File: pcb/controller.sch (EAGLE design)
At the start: 20 parts, among them J2 AVR_SPI_PROG_3X22X3_LOCK, Q1 ECS-160-20-3X-TR, U2 32U4

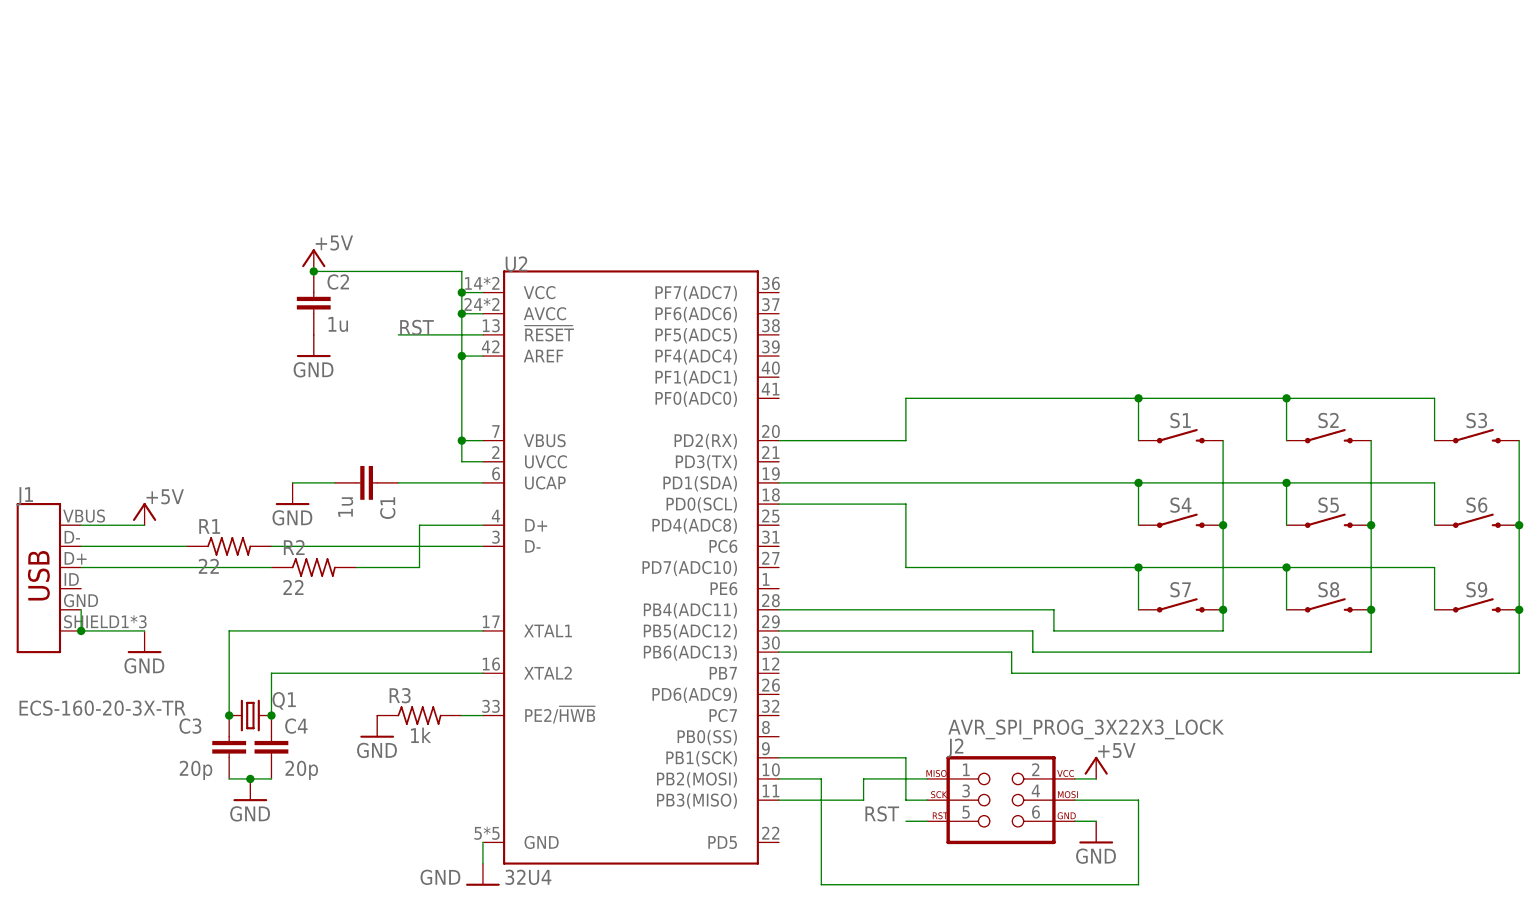
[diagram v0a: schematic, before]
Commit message: finish controller
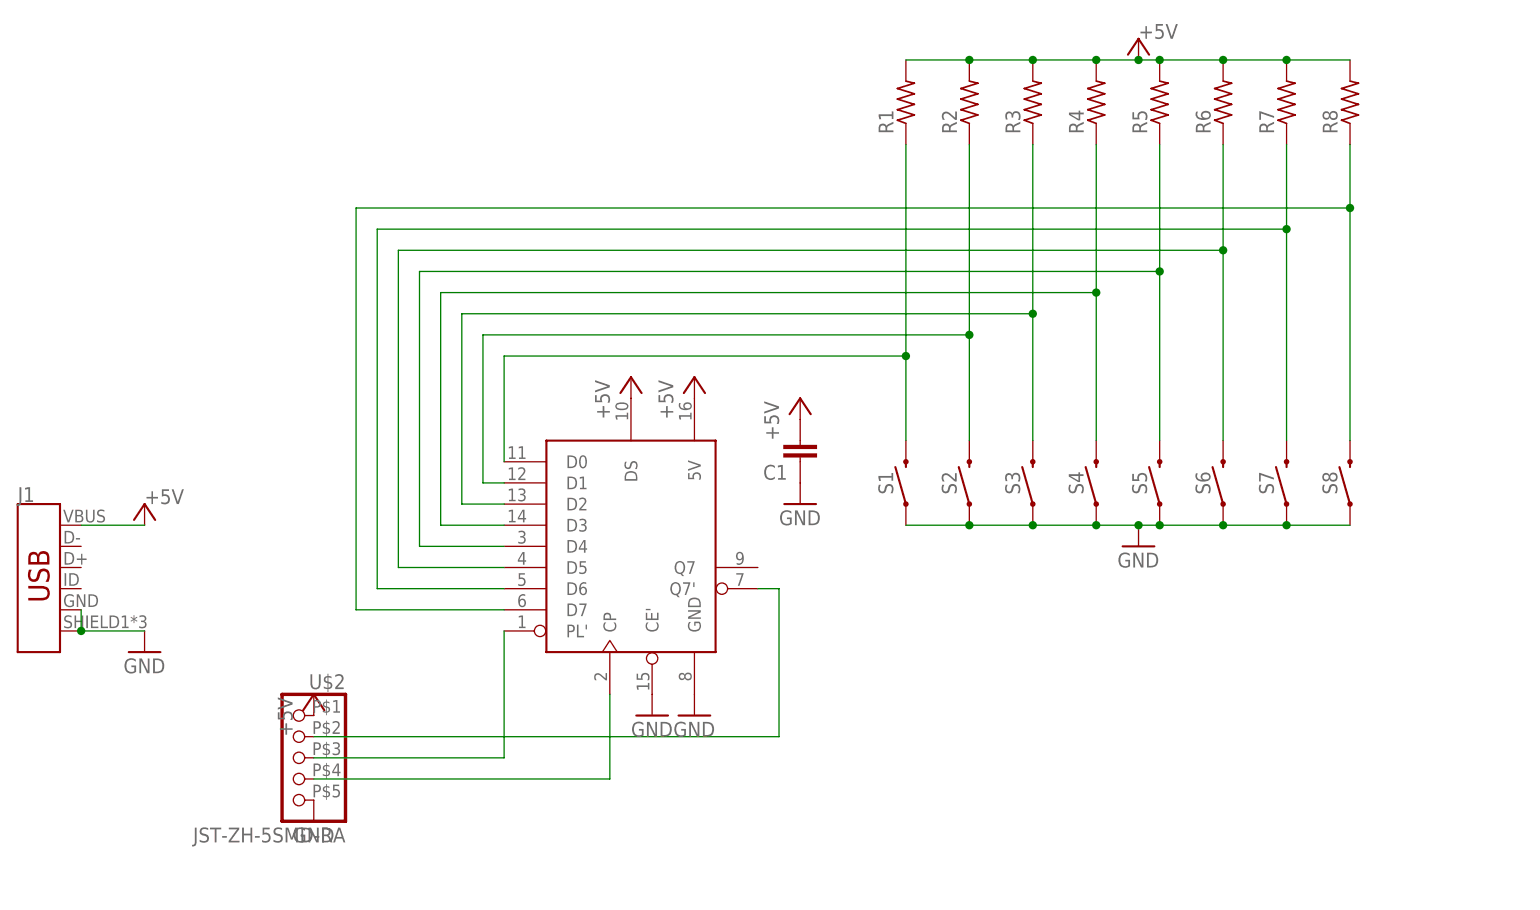
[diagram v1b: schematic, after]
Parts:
- removed C2: 1u, rcl:C-EUC0805
- removed C3, C4: 20p, rcl:C-EUC0805
- removed J2: AVR_SPI_PROG_3X22X3_LOCK, SparkFun-Connectors:AVR_SPI_PROG_3X22X3_LOCK
- removed Q1: ECS-160-20-3X-TR, adafruit:CRYSTALHC49UP
- removed S9: MOMENTARY-SWITCH-SPST-SMD-6.0X3.5MM, SparkFun-Switches:MOMENTARY-SWITCH-SPST-SMD-6.0X3.5MM
- removed U2: 32U4, SparkFun-IC-Microcontroller:ATMEGA32U4QFN
- added R4, R5, R6, R7, R8: (no value), rcl:R-US_R0603
- added U$2: JST-ZH-5SMD-RA, josh:JST-ZH-5SMD-RA
- added U1: 74HCT165TSSOP16, josh:74HCT165TSSOP16
- C1: value 1u -> (none); device rcl:C-EUC0805 -> rcl:C-EUC0603
- R1, R2: value 22 -> (none); device rcl:R-US_R0805 -> rcl:R-US_R0603
- R3: value 1k -> (none); device rcl:R-US_R0805 -> rcl:R-US_R0603
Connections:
- removed net N$12: S1.2, S4.2, S7.2, U2.PB4(ADC11)
- removed net N$13: S2.2, S5.2, S8.2, U2.PB5(ADC12)
- removed net N$14: S1.1, S2.1, S3.1, U2.PD2(RX)
- removed net N$18: S4.1, S5.1, S6.1, U2.PD1(SDA)
- removed net N$19: S3.2, S6.2, S9.2, U2.PB6(ADC13)
- removed net N$20: S7.1, S8.1, S9.1, U2.PD0(SCL)
- removed net RST: J2.5, U2.!RESET
- net +5V: now also C1.2, R1.2, R2.2, R3.2, R4.2, R5.2, R6.2, R7.2, R8.2, U$2.1, U1.5V, U1.DS; no longer C2.1, J2.2, U2.AREF, U2.AVCC@24, U2.UVCC, U2.VBUS, U2.VCC@14
- net GND: now also C1.1, S1.1, S2.1, S3.1, S4.1, S5.1, S6.1, S7.1, S8.1, U$2.5, U1.CE', U1.GND; no longer C1.2, C2.2, C3.2, C4.2, J2.6, R3.1, U2.GND
- net N$1: now also U$2.4, U1.CP; no longer C1.1, U2.UCAP
- net N$10: now also R7.1, S7.2, U1.D6; no longer J2.3, U2.PB1(SCK)
- net N$11: now also R8.1, S8.2, U1.D7; no longer J2.4, U2.PB2(MOSI)
- net N$2: now also U$2.3, U1.PL'; no longer J1.D-, R1.1
- net N$3: now also U$2.2, U1.Q7'; no longer J1.D+, R2.1
- net N$4: now also R1.1, S1.2, U1.D0; no longer R2.2, U2.D+
- net N$5: now also R2.1, S2.2, U1.D1; no longer R1.2, U2.D-
- net N$6: now also R3.1, S3.2, U1.D2; no longer R3.2, U2.PE2/!HWB
- net N$7: now also R4.1, S4.2, U1.D3; no longer C4.1, Q1.2, U2.XTAL2
- net N$8: now also R5.1, S5.2, U1.D4; no longer C3.1, Q1.1, U2.XTAL1
- net N$9: now also R6.1, S6.2, U1.D5; no longer J2.1, U2.PB3(MISO)
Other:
- moved on the sheet: C1, R1, R2, R3, S1, S2, S3, S4, S5, S6, S7, S8
